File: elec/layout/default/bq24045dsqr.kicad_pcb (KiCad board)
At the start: 2 copper layers, 225.7 x 100.8 mm, 8 parts

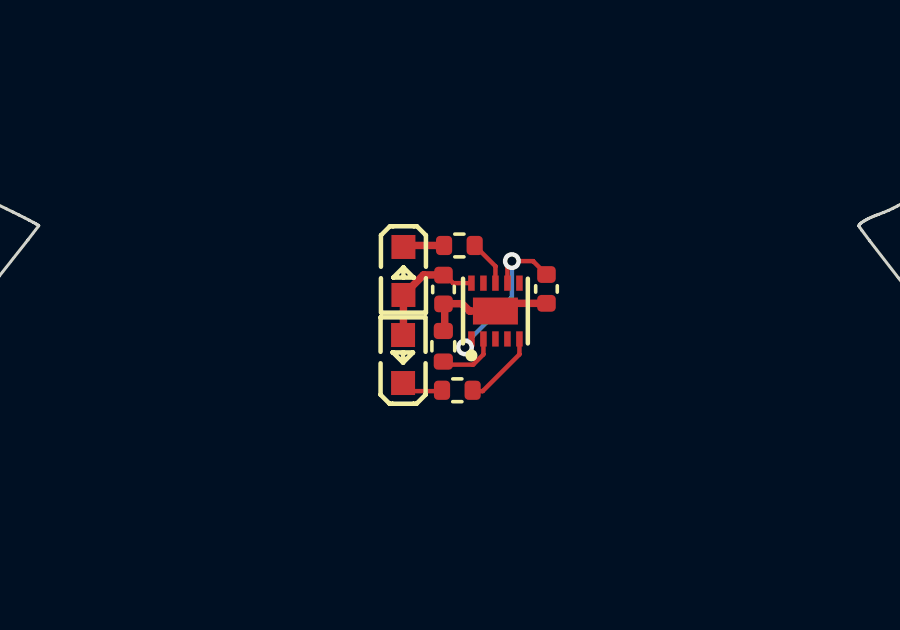
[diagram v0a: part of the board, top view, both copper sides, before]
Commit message: update layout
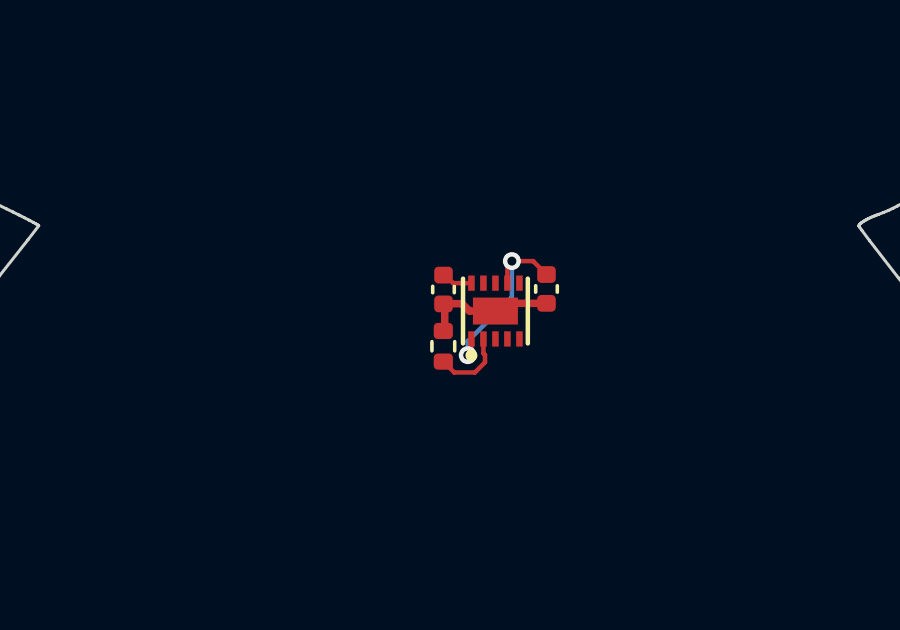
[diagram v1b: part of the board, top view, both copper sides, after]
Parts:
- removed LED1, LED2: , lib:LED0603-RD
- removed R2: Chip Resistor - Surface Mount 120Ohms ±5% 1/16W 0402 RoHS, lib:R0402
- removed R3: Chip Resistor - Surface Mount 82Ohms ±5% 1/16W 0402 RoHS, lib:R0402
- C1, C2: value Multilayer Ceramic Capacitors MLCC - SMD/SMT 1uF 6.3V 0402 RoHS -> 25V 1uF X5R ±10% 0402 Multilayer Ceramic Capacitors MLCC - SMD/SMT ROHS
- R1: value Chip Resistor - Surface Mount 560Ohms ±5% 1/16W 0402 RoHS -> 100mW Thick Film Resistors ±100ppm/℃ ±1% 604Ω 0402 Chip Resistor - Surface Mount ROHS
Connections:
- net gnd renamed ic-gnd
- net vcc renamed ic-vcc
- net vcc-1 renamed ic-vcc-1
- U1 pad 5: gnd-1 -> pg
- U1 pad 8: gnd-2 -> chg
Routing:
- net ic-vcc-1: track 4.16 -> 1.16 mm
- net gnd-1: track 2.53 -> 0.00 mm
- net gnd-2: track 1.55 -> 0.00 mm
- net cathode: track 1.46 -> 0.00 mm
- net cathode-1: track 1.38 -> 0.00 mm
- net iset: track 1.99 -> 2.76 mm
